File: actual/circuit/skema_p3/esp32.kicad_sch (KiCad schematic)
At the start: 35 parts, among them J1 Conn_01x04_Male, SW1 SW_Push, SW2 SW_Push, SW3 SW_Push, SW4 SW_Push, SW5 SW_Push, U1 ESP32-WROOM-32, U2 INMP441

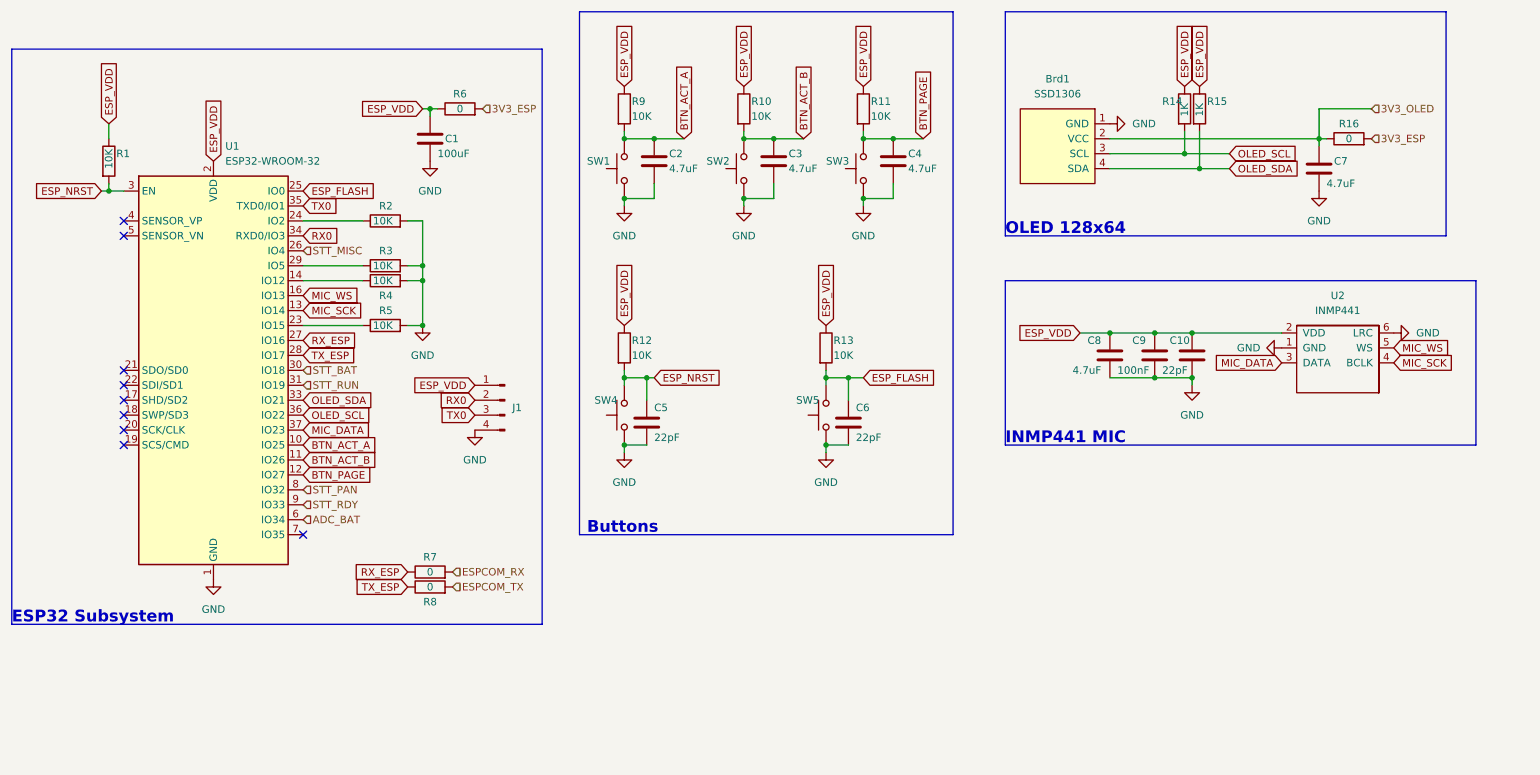
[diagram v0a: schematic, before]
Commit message: P3 in KiCAD
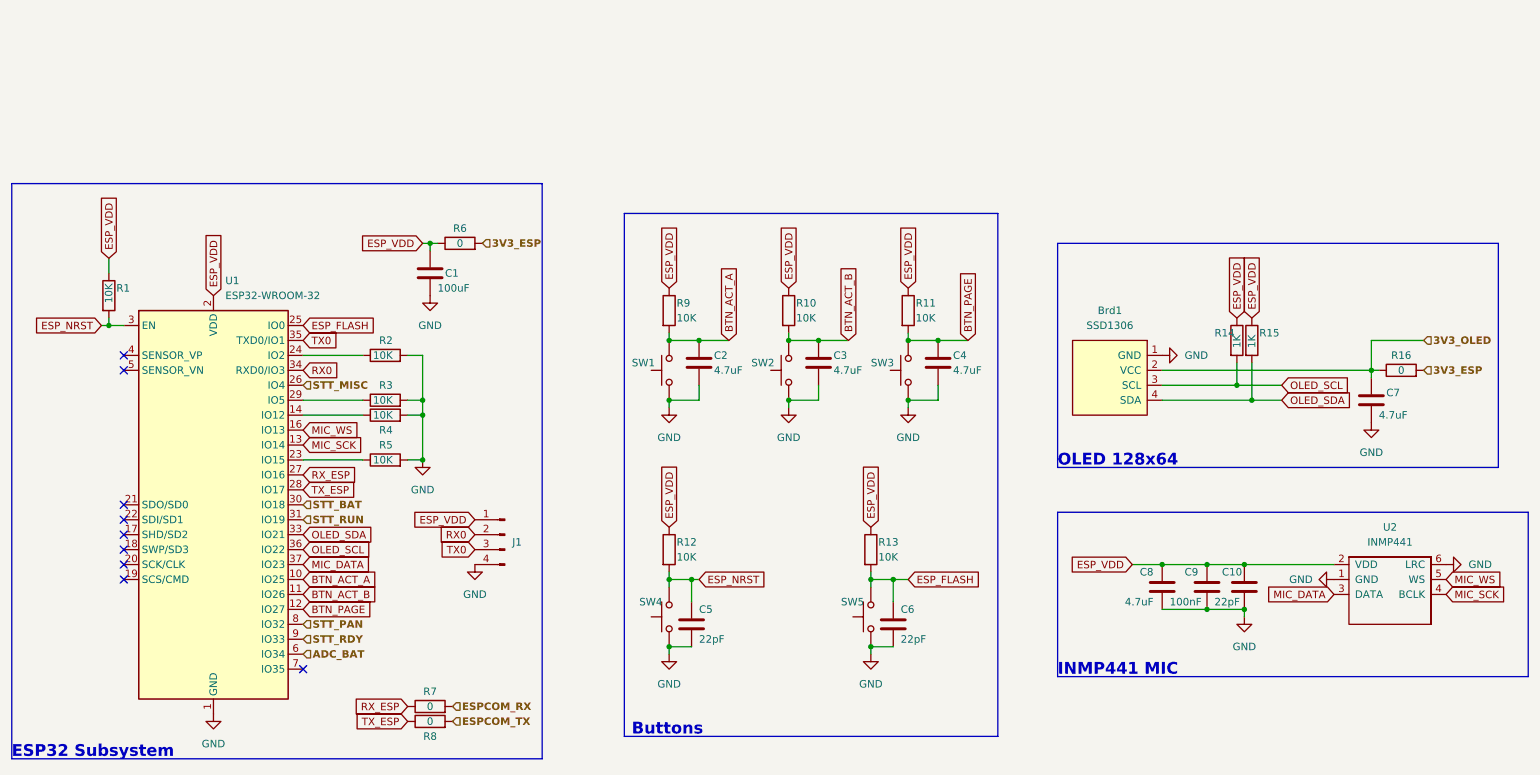
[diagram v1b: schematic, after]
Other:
- moved on the sheet: Brd1, C1, C10, C2, C3, C4, C5, C6, C7, C8, C9, J1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
